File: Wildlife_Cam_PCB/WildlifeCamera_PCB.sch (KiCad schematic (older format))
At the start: 47 parts, among them J1 PIR, J2 TRIG, J3 RTC_DS3231, J4 PROG, J5 PROG_EN, J6 LOGO1, J7 LOGO2, J8 PCB, J9 PV, Q1 2N3904, Q2 2N3904, Q3 BD135, SW1 ON/OFF, SW2 TRIGGER, U1 MCP1826S-3302, U2 BQ24210, U3 ESP32_CAM

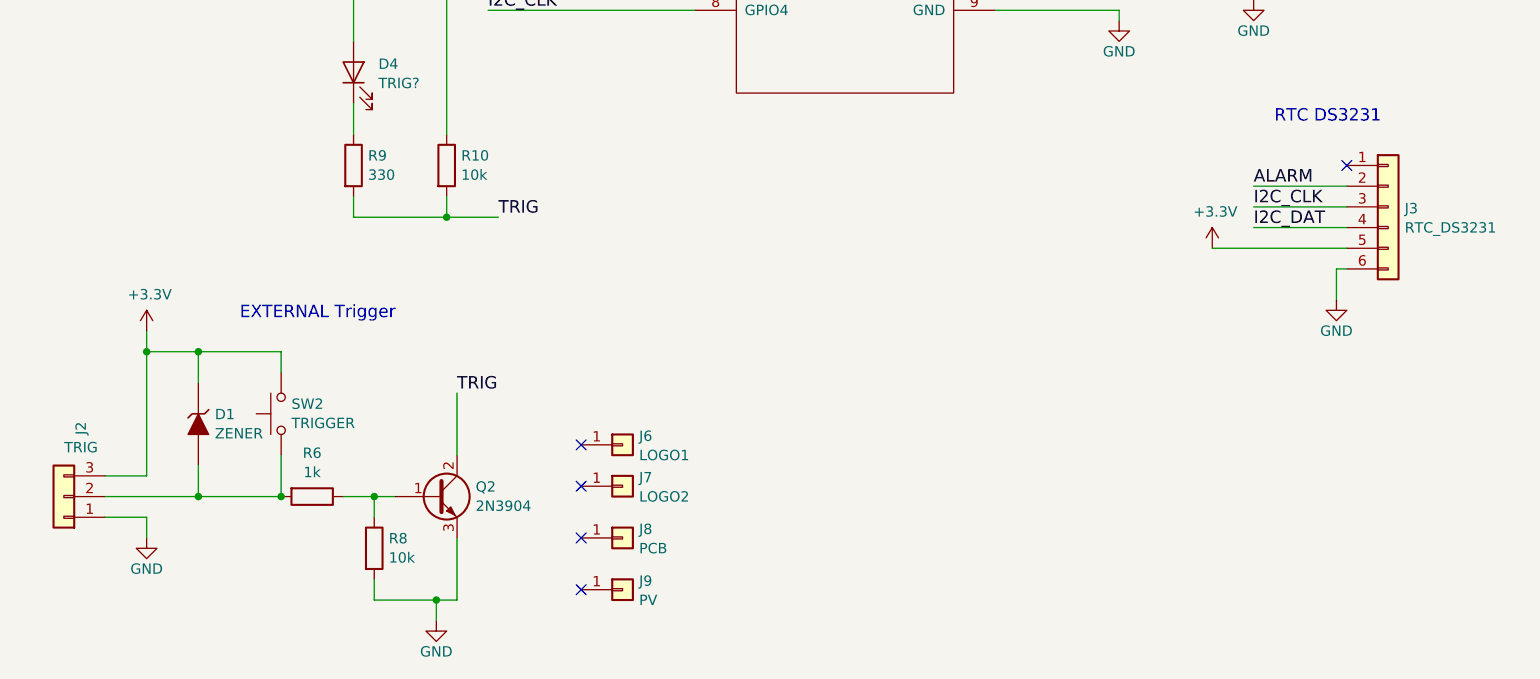
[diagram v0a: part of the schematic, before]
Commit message: Update of PCB
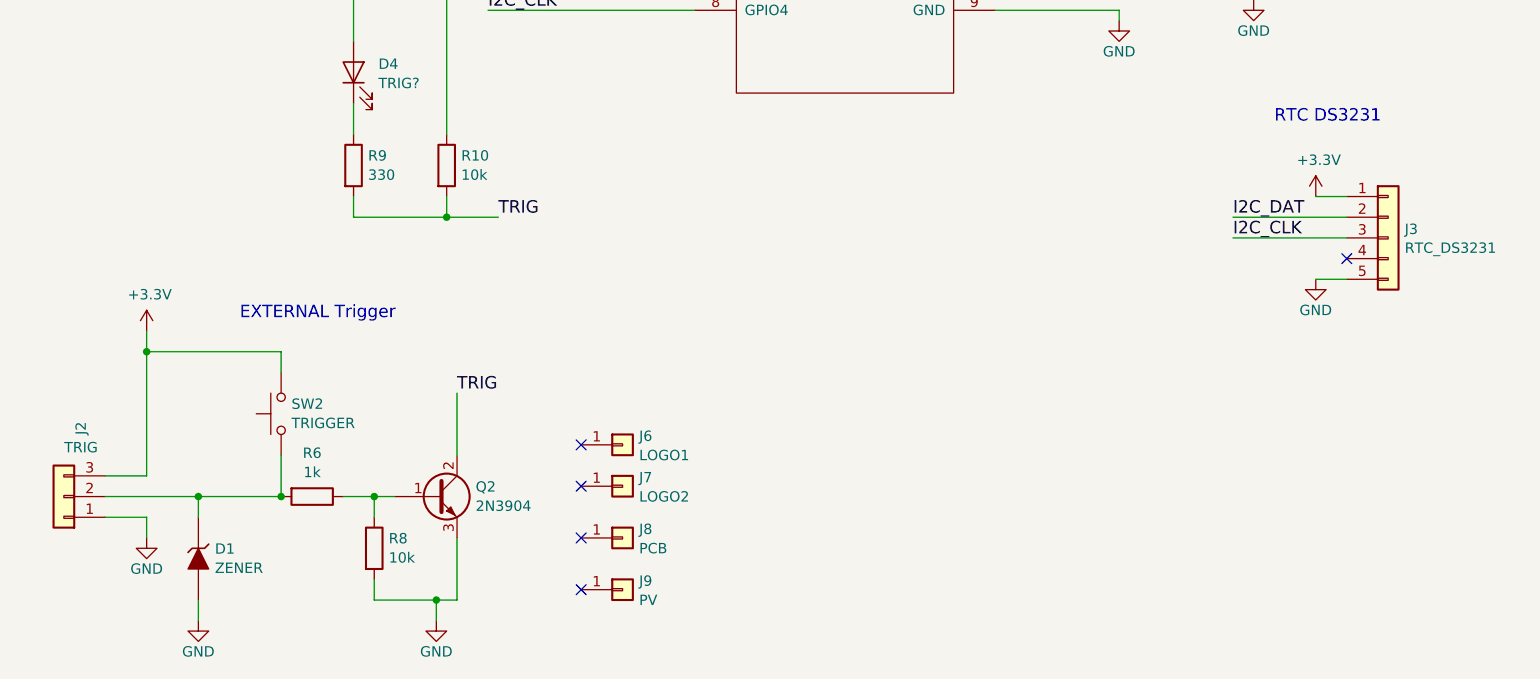
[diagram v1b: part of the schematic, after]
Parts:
- removed J3: RTC_DS3231, REInnovationFootprint:TH_RTC_MODULE, symbol WildlifeCamera_PCB-rescue:Conn_01x06-Connector_Generic
- added J3: RTC_DS3231, REInnovationFootprint:TH_RTC_MODULE_SM, symbol Connector_Generic:Conn_01x05
- J8: footprint (none) -> REInnovationFootprint:PCB_Wildlife_Cam
- Q3: footprint REInnovationFootprint:TO92-EBC_large_pad -> REInnovationFootprint:TO220_BD135
- SC1: footprint REInnovationFootprint:SIL-2_screw_terminal -> REInnovationFootprint:SIL_2_screw_+_JST_2mm
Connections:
- net +3V3: now also J3.1 (Pin_1); no longer D1.1 (K)
- net GND: now also D1.2 (A), J3.5 (Pin_5)
- net I2C_CLK: now also J3.3 (Pin_3)
- net I2C_DAT: now also J3.2 (Pin_2)
- net at J2.2 (Pin_2), R6.2, SW2.1: now also D1.1 (K); no longer D1.2 (A)
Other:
- moved on the sheet: D1
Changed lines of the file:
@@
 F 0 "SC1" H 950 1550 50  0000 L CNN
 F 1 "PV_IN" V 600 1350 50  0000 L CNN
-F 2 "REInnovationFootprint:SIL-2_screw_terminal" V 850 1510 50  0001 C CNN
+F 2 "REInnovationFootprint:SIL_2_screw_+_JST_2mm" V 850 1510 50  0001 C CNN
 F 3 "" V 850 1510 50  0000 C CNN
 F 4 "~" H 850 1450 60  0000 C CNN "Notes"
@@
 	4100 6850 4300 6850
 Wire Wire Line
-	4100 6950 4550 6950
-Wire Wire Line
-	4550 6950 4950 6950
-Connection ~ 4550 6950
-Wire Wire Line
 	5250 6950 5400 6950
 Wire Wire Line
@@
 Wire Wire Line
 	9700 3900 10150 3900
-$Comp
-L WildlifeCamera_PCB-rescue:+3.3V-power #PWR024
-U 1 1 5F57A570
-P 9450 5750
-F 0 "#PWR024" H 9450 5600 50  0001 C CNN
-F 1 "+3.3V" H 9465 5926 50  0000 C CNN
-F 2 "" H 9450 5750 50  0001 C CNN
-F 3 "" H 9450 5750 50  0001 C CNN
-	1    9450 5750
-	1    0    0    -1
-$EndComp
-$Comp
-L power1:GND #PWR027
-U 1 1 5F57ACA0
-P 10050 6000
-F 0 "#PWR027" H 10050 5750 50  0001 C CNN
-F 1 "GND" H 10050 5850 50  0000 C CNN
-F 2 "" H 10050 6000 50  0000 C CNN
-F 3 "" H 10050 6000 50  0000 C CNN
-	1    10050 6000
-	1    0    0    -1
-$EndComp
 Text Label 5950 4600 0    60   ~ 0
 I2C_CLK
 Text Label 5950 4500 0    60   ~ 0
 I2C_DAT
-Text Label 9650 5650 0    60   ~ 0
-I2C_DAT
-Text Label 9650 5550 0    60   ~ 0
-I2C_CLK
-Wire Wire Line
-	10100 5750 9450 5750
-Wire Wire Line
-	10100 5850 10050 5850
-Wire Wire Line
-	10050 5850 10050 6000
-Wire Wire Line
-	9650 5650 10100 5650
-Wire Wire Line
-	10100 5550 9650 5550
 Text Notes 9750 5150 0    60   ~ 0
 RTC DS3231
@@
 L matts_components:ZENER D1
 U 1 1 5F4F0673
-P 4550 6600
-F 0 "D1" V 4503 6680 50  0000 L CNN
-F 1 "ZENER" V 4596 6680 50  0000 L CNN
-F 2 "REInnovationFootprint:TH_Diode_3" H 4550 6600 50  0001 C CNN
-F 3 "" H 4550 6600 50  0000 C CNN
-	1    4550 6600
+P 4550 7250
+F 0 "D1" V 4503 7330 50  0000 L CNN
+F 1 "ZENER" V 4596 7330 50  0000 L CNN
+F 2 "REInnovationFootprint:TH_Diode_3" H 4550 7250 50  0001 C CNN
+F 3 "" H 4550 7250 50  0000 C CNN
+	1    4550 7250
 	0    1    1    0
 $EndComp
 Wire Wire Line
 	4950 6350 4950 6250
-Wire Wire Line
-	4950 6250 4550 6250
 Wire Wire Line
 	4300 6250 4300 6850
@@
 Connection ~ 4300 6250
 Wire Wire Line
-	4550 6400 4550 6250
-Connection ~ 4550 6250
-Wire Wire Line
-	4550 6250 4300 6250
-Wire Wire Line
 	4950 6750 4950 6950
 Connection ~ 4950 6950
-Wire Wire Line
-	4550 6800 4550 6950
-$Comp
-L WildlifeCamera_PCB-rescue:Conn_01x06-Connector_Generic J3
-U 1 1 5F510D1E
-P 10300 5550
-F 0 "J3" H 10380 5542 50  0000 L CNN
-F 1 "RTC_DS3231" H 10380 5449 50  0000 L CNN
-F 2 "REInnovationFootprint:TH_RTC_MODULE" H 10300 5550 50  0001 C CNN
-F 3 "~" H 10300 5550 50  0001 C CNN
-	1    10300 5550
-	1    0    0    -1
-$EndComp
 NoConn ~ 10150 3700
 NoConn ~ 10150 4100
-Text Label 9650 5450 0    60   ~ 0
-ALARM
-Wire Wire Line
-	9650 5450 10100 5450
-NoConn ~ 10100 5350
 $Comp
 L Connector_Generic:Conn_01x01 J7
@@
 F 0 "J8" H 6680 7192 50  0000 L CNN
 F 1 "PCB" H 6680 7099 50  0000 L CNN
-F 2 "" H 6600 7150 50  0001 C CNN
+F 2 "REInnovationFootprint:PCB_Wildlife_Cam" H 6600 7150 50  0001 C CNN
 F 3 "~" H 6600 7150 50  0001 C CNN
 	1    6600 7150
@@
 F 0 "Q3" H 1940 3597 50  0000 L CNN
 F 1 "BD135" H 1940 3504 50  0000 L CNN
-F 2 "REInnovationFootprint:TO92-EBC_large_pad" H 1950 3650 50  0001 C CNN
+F 2 "REInnovationFootprint:TO220_BD135" H 1950 3650 50  0001 C CNN
 F 3 "~" H 1750 3550 50  0001 C CNN
 	1    1750 3550
@@
 Wire Wire Line
 	8900 2250 8900 2200
+$Comp
+L Connector_Generic:Conn_01x05 J3
+U 1 1 5F9E542B
+P 10300 5700
+F 0 "J3" H 10380 5742 50  0000 L CNN
+F 1 "RTC_DS3231" H 10380 5651 50  0000 L CNN
+F 2 "REInnovationFootprint:TH_RTC_MODULE_SM" H 10300 5700 50  0001 C CNN
+F 3 "~" H 10300 5700 50  0001 C CNN
+	1    10300 5700
+	1    0    0    -1
+$EndComp
+$Comp
+L WildlifeCamera_PCB-rescue:+3.3V-power #PWR024
+U 1 1 5F9E59FA
+P 9950 5500
+F 0 "#PWR024" H 9950 5350 50  0001 C CNN
+F 1 "+3.3V" H 9965 5676 50  0000 C CNN
+F 2 "" H 9950 5500 50  0001 C CNN
+F 3 "" H 9950 5500 50  0001 C CNN
+	1    9950 5500
+	1    0    0    -1
+$EndComp
+$Comp
+L power1:GND #PWR027
+U 1 1 5F9E5C64
+P 9950 5900
+F 0 "#PWR027" H 9950 5650 50  0001 C CNN
+F 1 "GND" H 9950 5750 50  0000 C CNN
+F 2 "" H 9950 5900 50  0000 C CNN
+F 3 "" H 9950 5900 50  0000 C CNN
+	1    9950 5900
+	1    0    0    -1
+$EndComp
+Text Label 9550 5700 0    60   ~ 0
+I2C_CLK
+Text Label 9550 5600 0    60   ~ 0
+I2C_DAT
+NoConn ~ 10100 5800
+Wire Wire Line
+	10100 5900 9950 5900
+Wire Wire Line
+	9950 5500 10100 5500
+Wire Wire Line
+	10100 5600 9550 5600
+Wire Wire Line
+	9550 5700 10100 5700
+Wire Wire Line
+	4100 6950 4550 6950
+Wire Wire Line
+	4300 6250 4950 6250
+Wire Wire Line
+	4550 7050 4550 6950
+Connection ~ 4550 6950
+Wire Wire Line
+	4550 6950 4950 6950
+$Comp
+L power1:GND #PWR0101
+U 1 1 5FA7F2FD
+P 4550 7550
+F 0 "#PWR0101" H 4550 7300 50  0001 C CNN
+F 1 "GND" H 4550 7400 50  0000 C CNN
+F 2 "" H 4550 7550 50  0000 C CNN
+F 3 "" H 4550 7550 50  0000 C CNN
+	1    4550 7550
+	1    0    0    -1
+$EndComp
+Wire Wire Line
+	4550 7550 4550 7450
 $EndSCHEMATC
